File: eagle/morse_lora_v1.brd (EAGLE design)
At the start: 68.6 x 83.4 mm, 20 parts

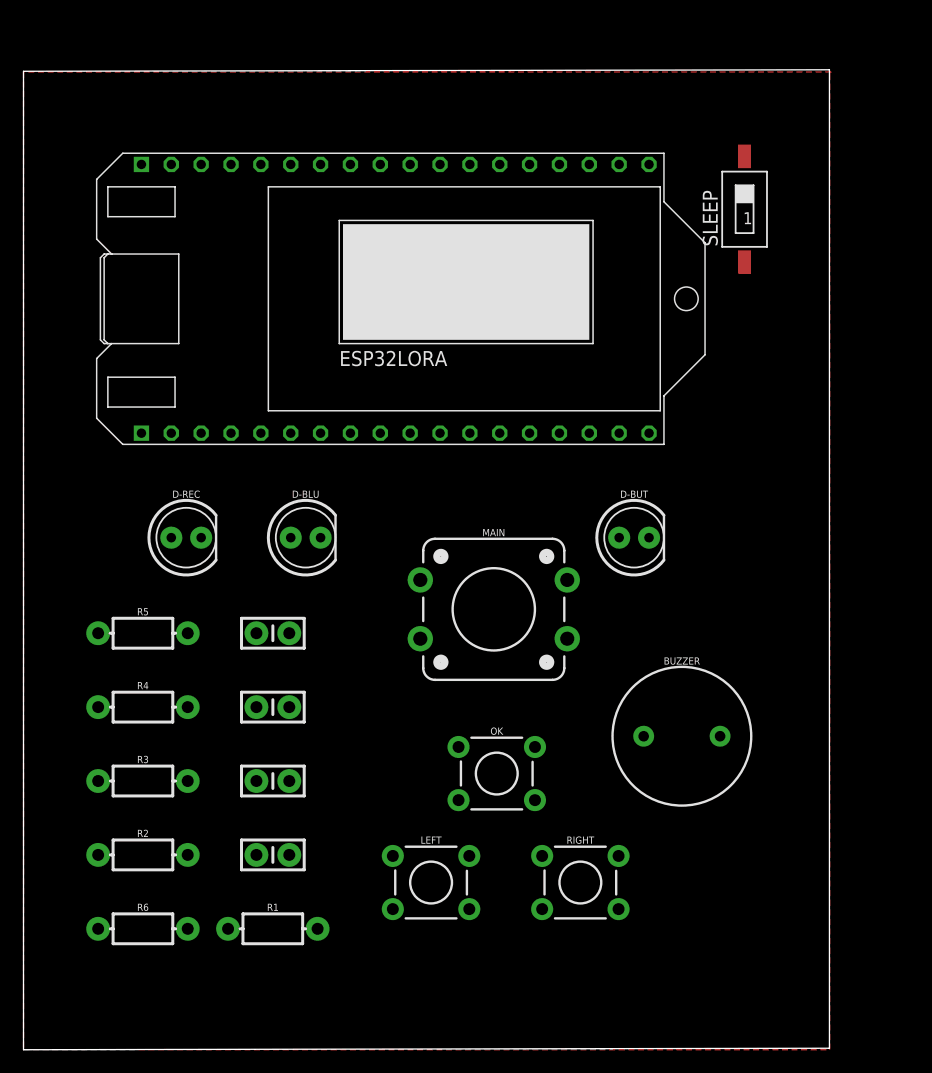
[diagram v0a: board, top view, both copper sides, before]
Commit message: draft layout
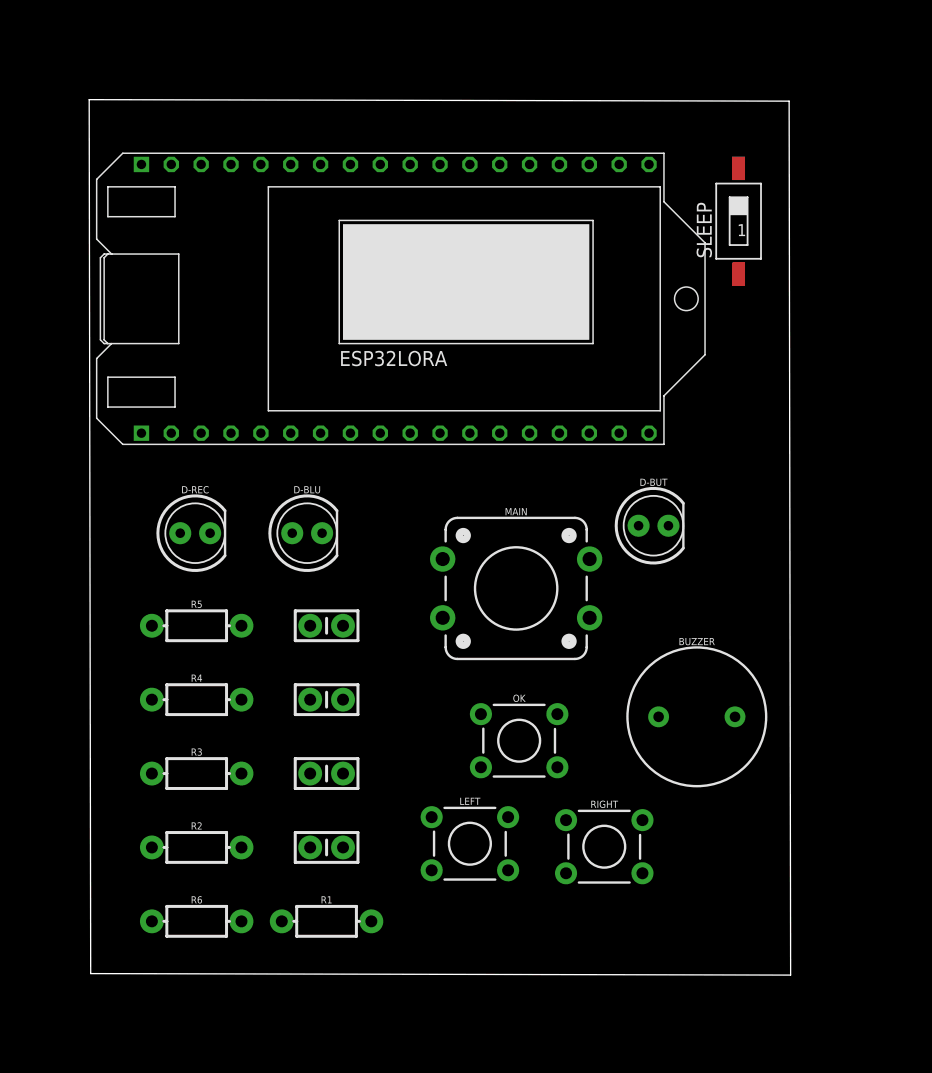
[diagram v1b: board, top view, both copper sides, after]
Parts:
- moved LEFT 4.67 mm to (66.0, 33.7)
- moved C1 4.62 mm to (53.9, 52.2)
- moved C3 4.62 mm to (53.9, 39.6)
- moved R3 4.62 mm to (42.8, 39.6)
- moved R5 4.62 mm to (42.8, 52.2)
- moved C2 4.62 mm to (53.9, 45.9)
- moved C4 4.62 mm to (53.9, 33.3)
- moved R2 4.62 mm to (42.8, 33.3)
- moved R4 4.62 mm to (42.8, 45.9)
- moved R6 4.62 mm to (42.8, 27.1)
- moved R1 4.62 mm to (53.8, 27.1)
- moved RIGHT 3.66 mm to (77.5, 33.4)
- moved OK 3.38 mm to (70.2, 42.4)
- moved MAIN 2.61 mm to (70.0, 55.4)
- moved BUZZER 2.08 mm to (85.3, 44.5)
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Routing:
- removed copper zone on layer 1, net GND
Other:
- board size 68.6 x 83.4 mm -> 59.7 x 74.5 mm

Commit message: draft layout
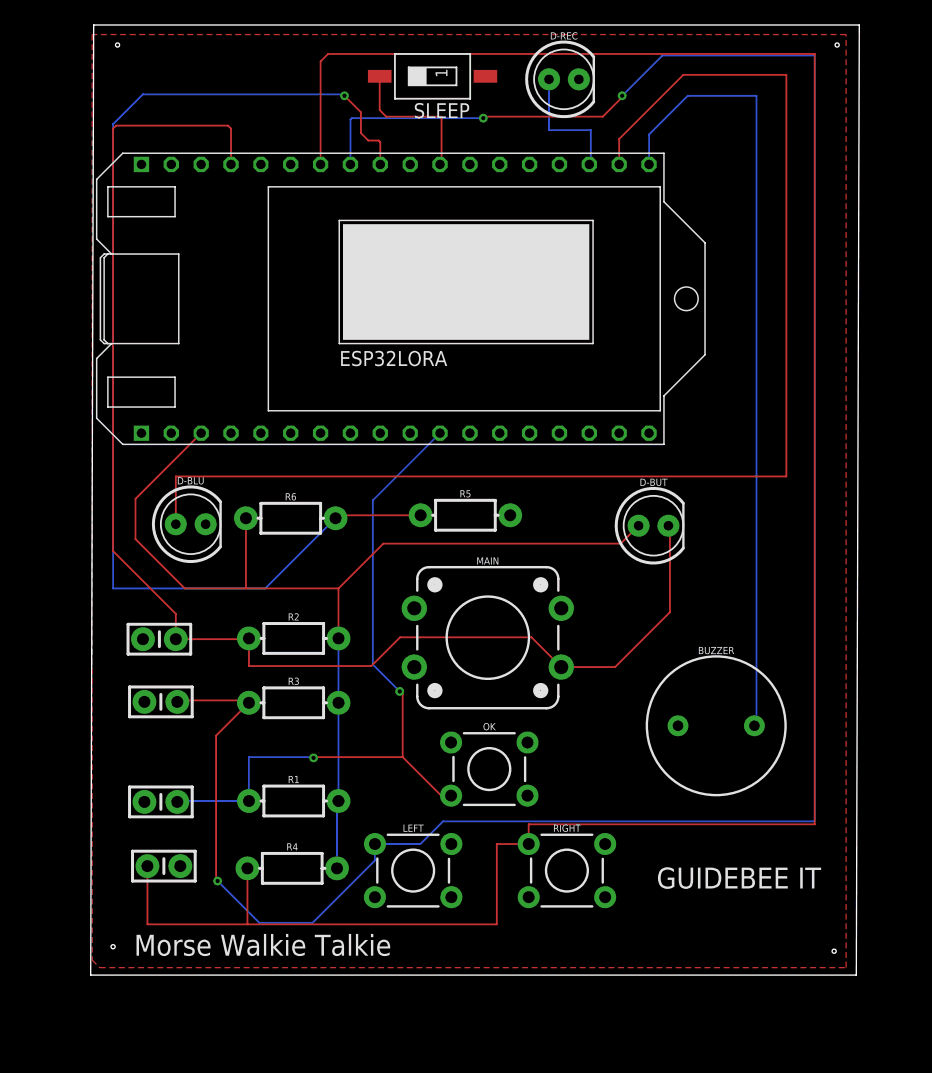
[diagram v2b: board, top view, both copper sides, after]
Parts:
- moved D-REC 49.7 mm to (74.0, 98.7)
- moved R6 35.2 mm to (50.8, 61.3)
- moved SLEEP 28.8 mm to (62.9, 98.9), turned to 90 degrees
- moved R5 24.7 mm to (65.7, 61.6)
- moved R2 19.6 mm to (51.1, 51.1)
- moved R4 16.5 mm to (50.9, 31.6)
- moved C3 15.9 mm to (40.0, 31.8)
- moved C4 14.6 mm to (39.8, 37.2)
- moved C1 14.3 mm to (39.6, 51.1)
- moved C2 14.1 mm to (39.8, 45.7)
- moved R1 10.6 mm to (51.1, 37.3)
- moved R3 10.2 mm to (51.1, 45.6)
- moved D-BLU 9.94 mm to (42.3, 60.8)
- moved LEFT 5.34 mm to (61.2, 31.4)
- moved MAIN 4.84 mm to (67.6, 51.2)
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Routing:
- net 39: track 0.00 -> 191.6 mm
- net 34: track 0.00 -> 190.3 mm, vias 0 -> 3
- net 36: track 0.00 -> 114.8 mm
- net N$6: track 0.00 -> 108.8 mm
- net 35: track 0.00 -> 96.7 mm, vias 0 -> 1
- net 3V3: track 0.00 -> 87.9 mm
- net N$4: track 0.00 -> 66.8 mm
- net 23: track 0.00 -> 59.5 mm, vias 0 -> 2
- net N$13: track 0.00 -> 12.5 mm
- net N$5: track 0.00 -> 10.8 mm
- added copper zone on layer 1, net GND
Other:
- board size 59.7 x 74.5 mm -> 65.4 x 80.8 mm
- board text added: "GUIDEBEE IT"
- board text added: "Morse Walkie Talkie"

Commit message: update pcb v1
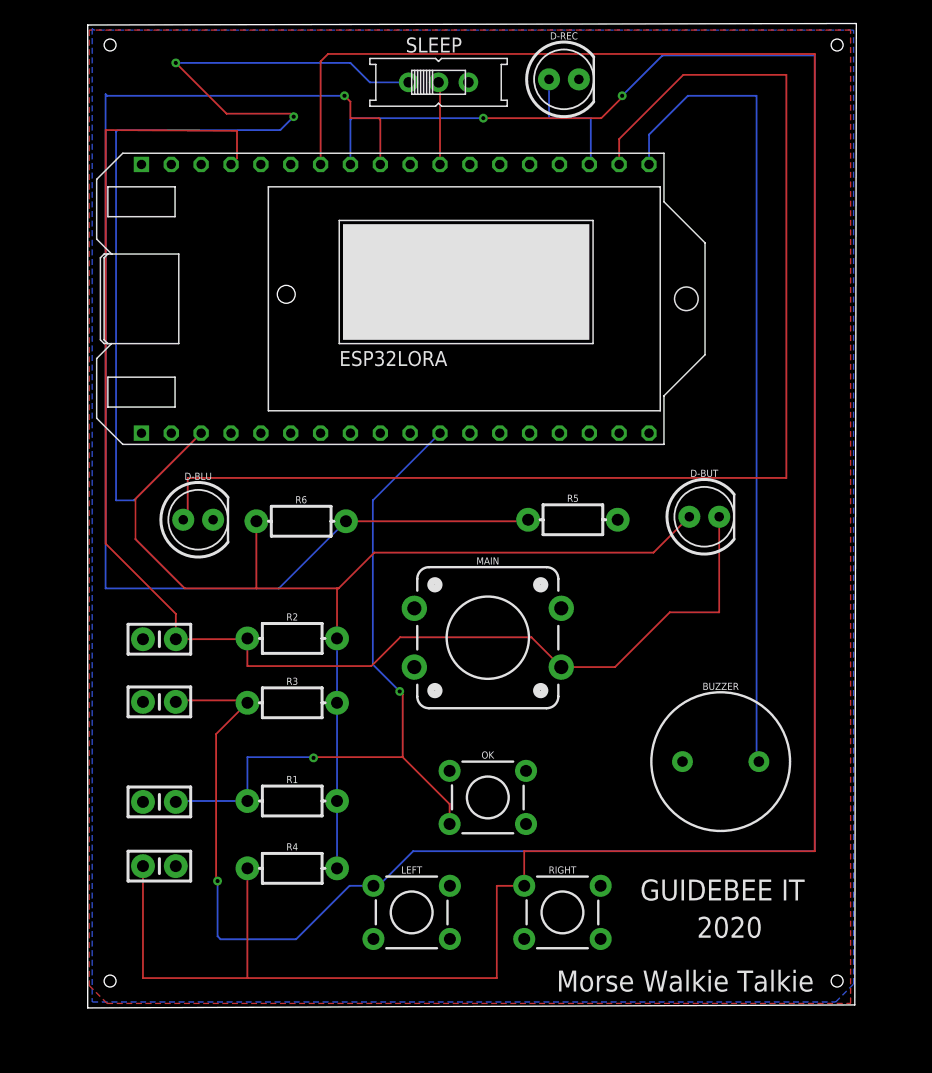
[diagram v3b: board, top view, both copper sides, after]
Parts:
- SLEEP: value SWS001 -> (none); device smd-special:SMS-001 -> adafruit:EG1218
- moved R5 9.15 mm to (74.8, 61.2)
- moved D-BUT 4.38 mm to (86.0, 61.5)
- moved RIGHT 3.58 mm to (73.9, 27.8)
- moved LEFT 3.56 mm to (61.1, 27.8)
- moved BUZZER 3.07 mm to (87.4, 40.6)
- moved OK 2.42 mm to (67.6, 37.6)
- moved R6 0.92 mm to (51.7, 61.1)
- moved D-BLU 0.74 mm to (42.9, 61.2)
- moved SLEEP 0.72 mm to (63.4, 98.4), turned to 0 degrees
- moved C3 0.38 mm to (39.6, 31.8)
- moved R1 0.13 mm to (50.9, 37.3)
- moved R2 0.13 mm to (50.9, 51.1)
- moved R3 0.13 mm to (50.9, 45.6)
- moved C2 0.13 mm to (39.6, 45.7)
- moved C4 0.13 mm to (39.6, 37.2)
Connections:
- net 3V3: now also SLEEP.O
- net GND: now also ESP32LORA.P$1, SLEEP.S; no longer SLEEP.1
- net N$13: now also SLEEP.P; no longer SLEEP.2
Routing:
- net 3V3: track 87.9 -> 181.3 mm, vias 0 -> 2
- net 39: track 191.6 -> 205.7 mm
- net 35: track 96.7 -> 109.3 mm
- net 36: track 114.8 -> 120.8 mm
- net N$13: track 12.5 -> 7.04 mm
- net 34: track 190.3 -> 194.7 mm
- net N$4: track 66.8 -> 69.9 mm
- net 23: track 59.5 -> 61.5 mm
- net N$6: track 108.8 -> 107.6 mm
- added copper zone on layer 16, net GND
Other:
- board size 65.4 x 80.8 mm -> 65.4 x 83.7 mm
- board text added: "2020"

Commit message: update pcb v2
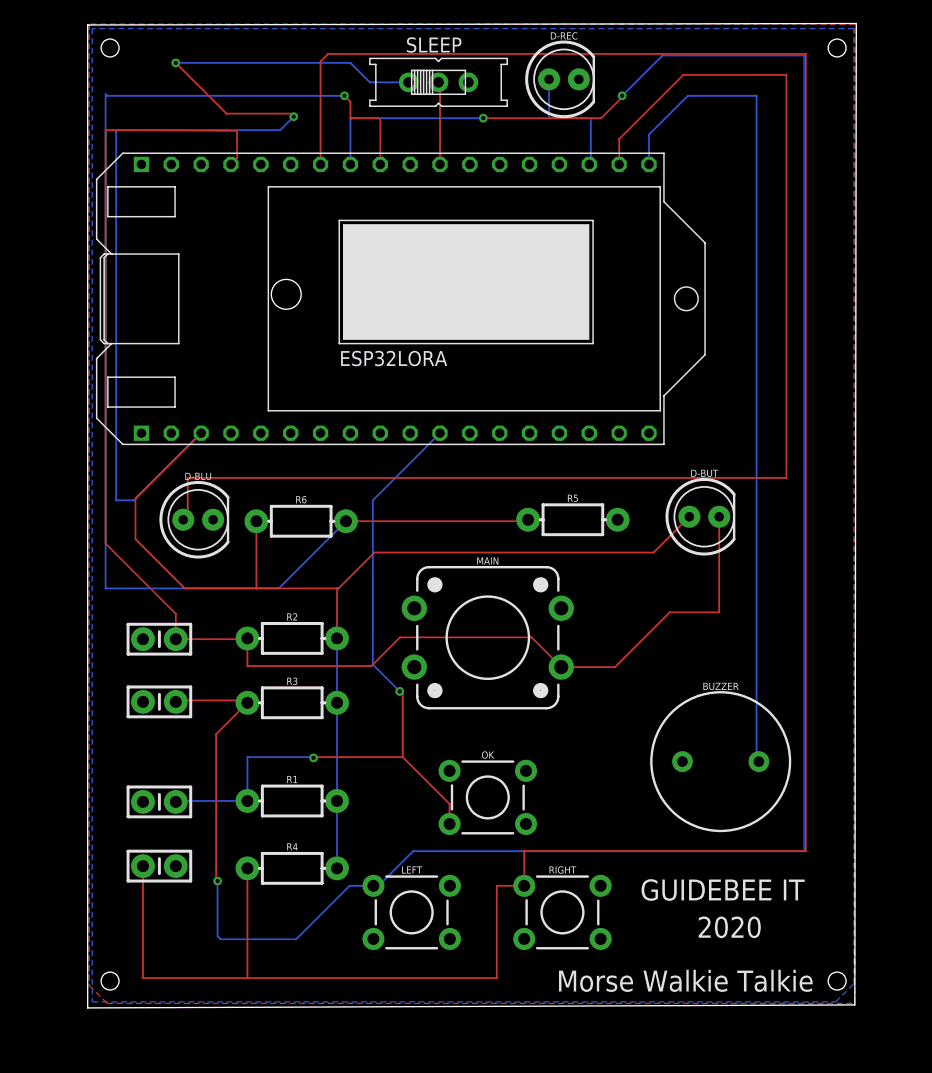
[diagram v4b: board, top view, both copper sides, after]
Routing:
- net 34: track 194.7 -> 192.9 mm
- net 39: track 205.7 -> 204.2 mm
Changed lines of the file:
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@@
 <wire x1="98.913" y1="103.429" x2="33.528" y2="103.302" width="0" layer="20"/>
 <wire x1="33.528" y1="103.302" x2="33.528" y2="19.685" width="0" layer="20"/>
-<hole x="35.433" y="101.6" drill="1.016"/>
-<hole x="97.282" y="101.6" drill="1.016" grouprefs="HOLES"/>
-<hole x="97.282" y="21.971" drill="1.016" grouprefs="HOLES"/>
-<hole x="35.433" y="21.971" drill="1.016" grouprefs="HOLES"/>
+<hole x="35.433" y="101.346" drill="1.524"/>
+<hole x="97.282" y="101.346" drill="1.524" grouprefs="HOLES"/>
+<hole x="97.282" y="21.971" drill="1.524" grouprefs="HOLES"/>
+<hole x="35.433" y="21.971" drill="1.524" grouprefs="HOLES"/>
 <text x="73.406" y="21.082" size="1.778" layer="25">Morse Walkie Talkie</text>
 <text x="80.518" y="28.829" size="1.778" layer="25">GUIDEBEE IT</text>
-<hole x="50.419" y="80.391" drill="1.524"/>
+<hole x="50.419" y="80.391" drill="2.54"/>
 <text x="85.344" y="25.654" size="1.778" layer="25">2020</text>
 </plain>
@@
 <contactref element="BUZZER" pad="-"/>
 <polygon width="0.1524" layer="1">
-<vertex x="33.655" y="102.87"/>
+<vertex x="33.655" y="103.378"/>
 <vertex x="33.655" y="21.59"/>
 <vertex x="35.179" y="20.066"/>
-<vertex x="98.425" y="20.066"/>
-<vertex x="98.425" y="102.87"/>
+<vertex x="98.806" y="20.066"/>
+<vertex x="98.806" y="103.378"/>
 </polygon>
 <contactref element="ESP32LORA" pad="P$1"/>
@@
 <vertex x="33.909" y="20.193"/>
 <vertex x="97.155" y="20.193"/>
-<vertex x="98.679" y="21.717"/>
-<vertex x="98.679" y="102.87"/>
-<vertex x="34.036" y="102.87"/>
+<vertex x="98.71075" y="21.74875"/>
+<vertex x="98.71075" y="102.997"/>
 </polygon>
 </signal>
@@
 <contactref element="C3" pad="1"/>
 <contactref element="RIGHT" pad="1"/>
-<wire x1="95.377" y1="33.02" x2="95.377" y2="100.838" width="0.1524" layer="1"/>
+<wire x1="94.615" y1="33.02" x2="94.615" y2="100.838" width="0.1524" layer="1"/>
 <wire x1="53.975" y1="100.838" x2="53.34" y2="100.203" width="0.1524" layer="1"/>
 <wire x1="53.34" y1="100.203" x2="53.34" y2="91.44" width="0.1524" layer="1"/>
-<wire x1="70.6628" y1="33.02" x2="95.377" y2="33.02" width="0.1524" layer="1"/>
-<wire x1="95.377" y1="100.838" x2="53.975" y2="100.838" width="0.1524" layer="1"/>
+<wire x1="70.6628" y1="33.02" x2="94.615" y2="33.02" width="0.1524" layer="1"/>
+<wire x1="94.615" y1="100.838" x2="53.975" y2="100.838" width="0.1524" layer="1"/>
 <wire x1="70.6628" y1="30.0736" x2="68.326" y2="30.0736" width="0.1524" layer="1"/>
 <wire x1="68.326" y1="30.0736" x2="68.326" y2="22.225" width="0.1524" layer="1"/>
@@
 <wire x1="57.8358" y1="30.0736" x2="58.2676" y2="30.0736" width="0.1524" layer="16"/>
 <wire x1="58.2676" y1="30.0736" x2="61.214" y2="33.02" width="0.1524" layer="16"/>
-<wire x1="61.214" y1="33.02" x2="95.377" y2="33.02" width="0.1524" layer="16"/>
-<wire x1="95.377" y1="33.02" x2="95.377" y2="100.711" width="0.1524" layer="16"/>
-<wire x1="95.377" y1="100.711" x2="82.423" y2="100.711" width="0.1524" layer="16"/>
+<wire x1="61.214" y1="33.02" x2="94.488" y2="33.02" width="0.1524" layer="16"/>
+<wire x1="94.488" y1="33.02" x2="94.488" y2="100.711" width="0.1524" layer="16"/>
+<wire x1="94.488" y1="100.711" x2="82.423" y2="100.711" width="0.1524" layer="16"/>
 <wire x1="82.423" y1="100.711" x2="78.994" y2="97.282" width="0.1524" layer="16"/>
 <via x="78.994" y="97.282" extent="1-16" drill="0.35"/>
